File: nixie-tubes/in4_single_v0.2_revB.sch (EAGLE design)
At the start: 15 parts, among them IC1 74HC595D, IC2 74HC595D, IC3 ULN2003AD, IC4 ULN2003AD

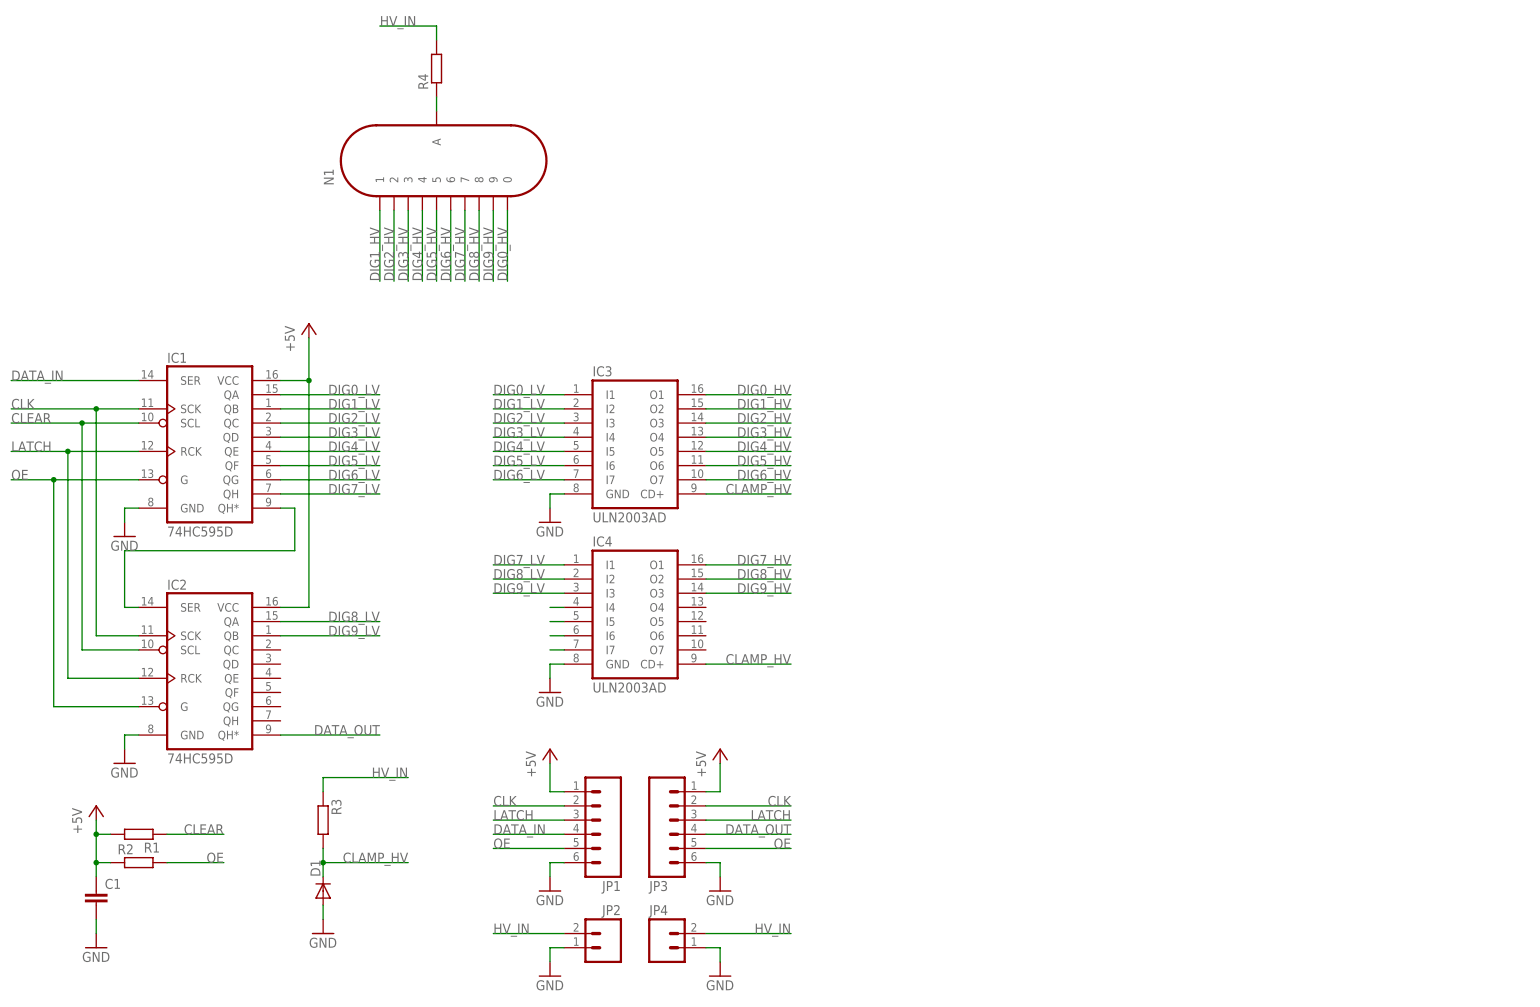
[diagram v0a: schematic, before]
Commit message: cleanup, schematic, footprint change
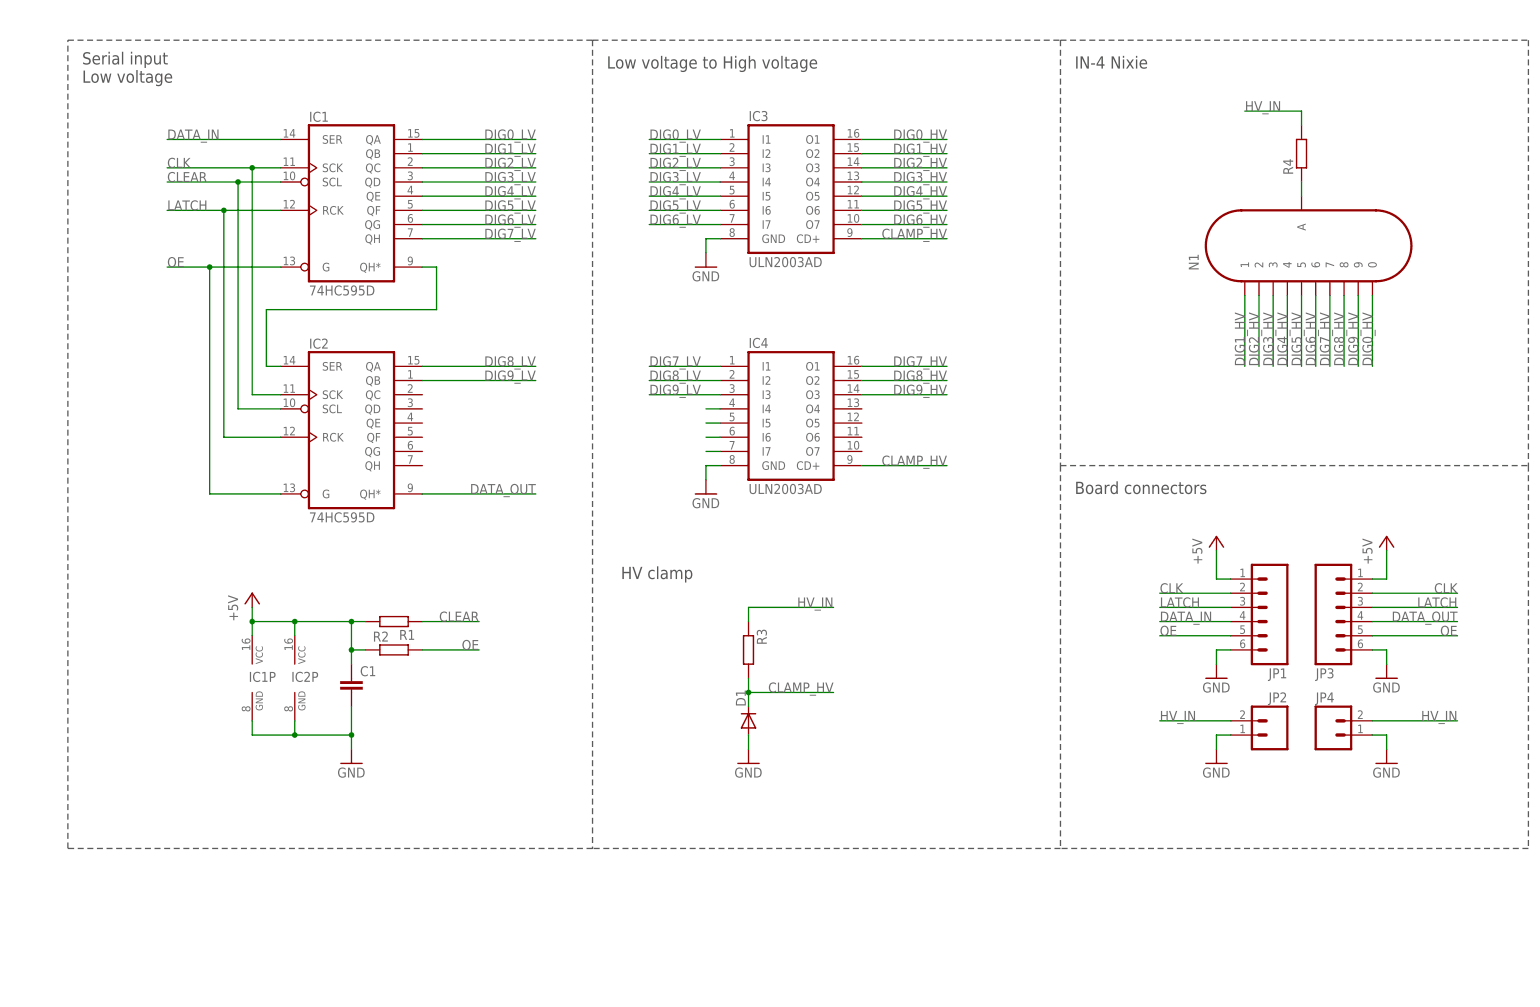
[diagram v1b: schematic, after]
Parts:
- IC1: device SparkFun-DigitalIC:74LS595D -> 74xx-eu:74HC595D
- IC2: device SparkFun-DigitalIC:74LS595D -> 74xx-eu:74HC595D; PROD_ID IC-07875 -> (none)
- R4: device resistor:R-EU_R1206 -> resistor:R-EU_R1210
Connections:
- net +5V: now also IC1P.VCC, IC2P.VCC; no longer IC1.VCC, IC2.VCC
- net CLEAR: now also IC1A.SCL, IC2A.SCL; no longer IC1.SCL, IC2.SCL
- net CLK: now also IC1A.SCK, IC2A.SCK; no longer IC1.SCK, IC2.SCK
- net DATA_IN: now also IC1A.SER; no longer IC1.SER
- net DATA_OUT: now also IC2A.QH*; no longer IC2.QH*
- net DIG0_LV: now also IC1A.QA; no longer IC1.QA
- net DIG1_LV: now also IC1A.QB; no longer IC1.QB
- net DIG2_LV: now also IC1A.QC; no longer IC1.QC
- net DIG3_LV: now also IC1A.QD; no longer IC1.QD
- net DIG4_LV: now also IC1A.QE; no longer IC1.QE
- net DIG5_LV: now also IC1A.QF; no longer IC1.QF
- net DIG6_LV: now also IC1A.QG; no longer IC1.QG
- net DIG7_LV: now also IC1A.QH; no longer IC1.QH
- net DIG8_LV: now also IC2A.QA; no longer IC2.QA
- net DIG9_LV: now also IC2A.QB; no longer IC2.QB
- net GND: now also IC1P.GND, IC2P.GND; no longer IC1.GND, IC2.GND
- net LATCH: now also IC1A.RCK, IC2A.RCK; no longer IC1.RCK, IC2.RCK
- net N$1: now also IC1A.QH*, IC2A.SER; no longer IC1.QH*, IC2.SER
- net OE: now also IC1A.G, IC2A.G; no longer IC1.G, IC2.G
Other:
- note added: "Board connectors"
- note added: "HV clamp"
- note added: "IN-4 Nixie"
- note added: "Low voltage to High voltage"
- note added: "Serial input Low voltage"
- moved on the sheet: C1, D1, IC3, IC4, JP1, JP2, JP3, JP4, N1, R1, R2, R3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
